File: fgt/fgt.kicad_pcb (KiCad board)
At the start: 2 copper layers, 78 x 78 mm, 60 parts, among them J1 Conn_01x02, J2 USB_B_Mini, J3 BL_Conn, J4 Conn_01x06, Q1 BC817, SW1 Reset, SW2 SW-, SW3 SW_M/BOOT, SW4 SW+, U1 ESP32-C3-WROOM-02, U2 ERC12864, U3 BMP280, U4 HT75xx-1-SOT89

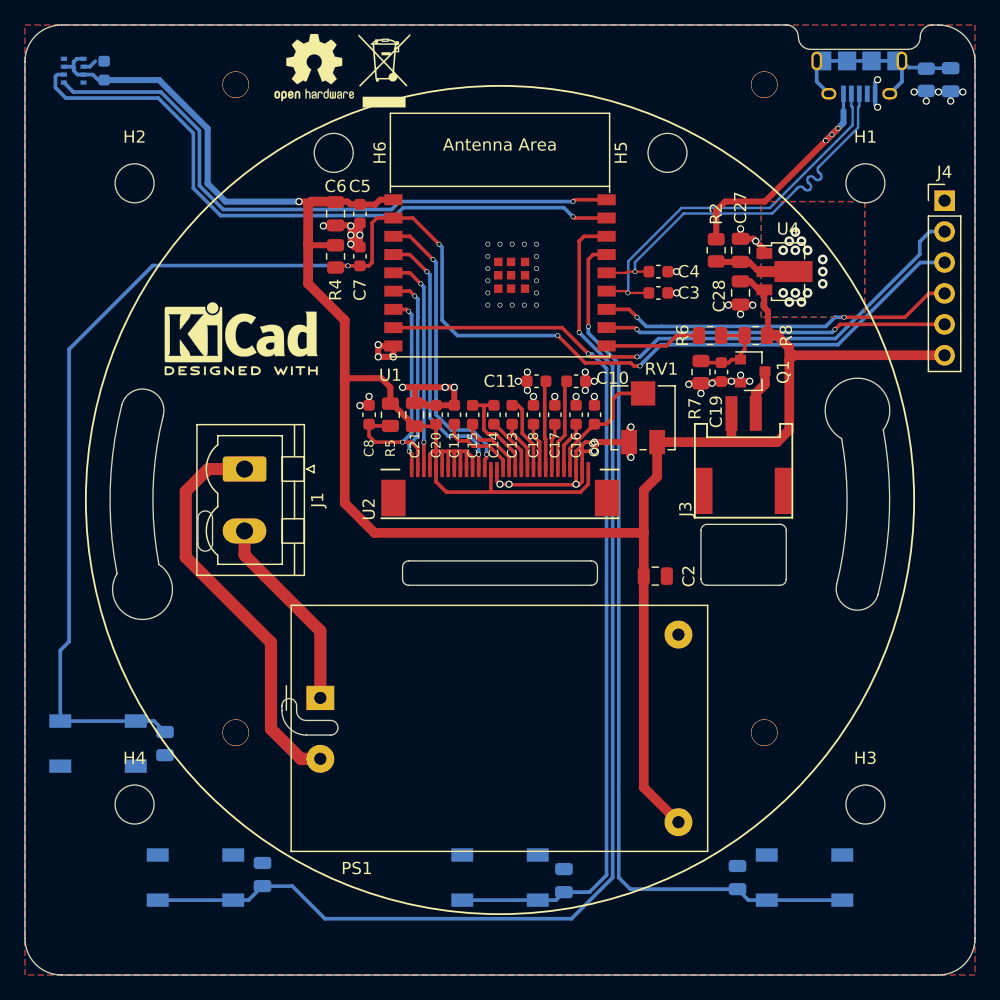
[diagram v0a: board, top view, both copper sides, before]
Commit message: retouch board layout v1.1.0
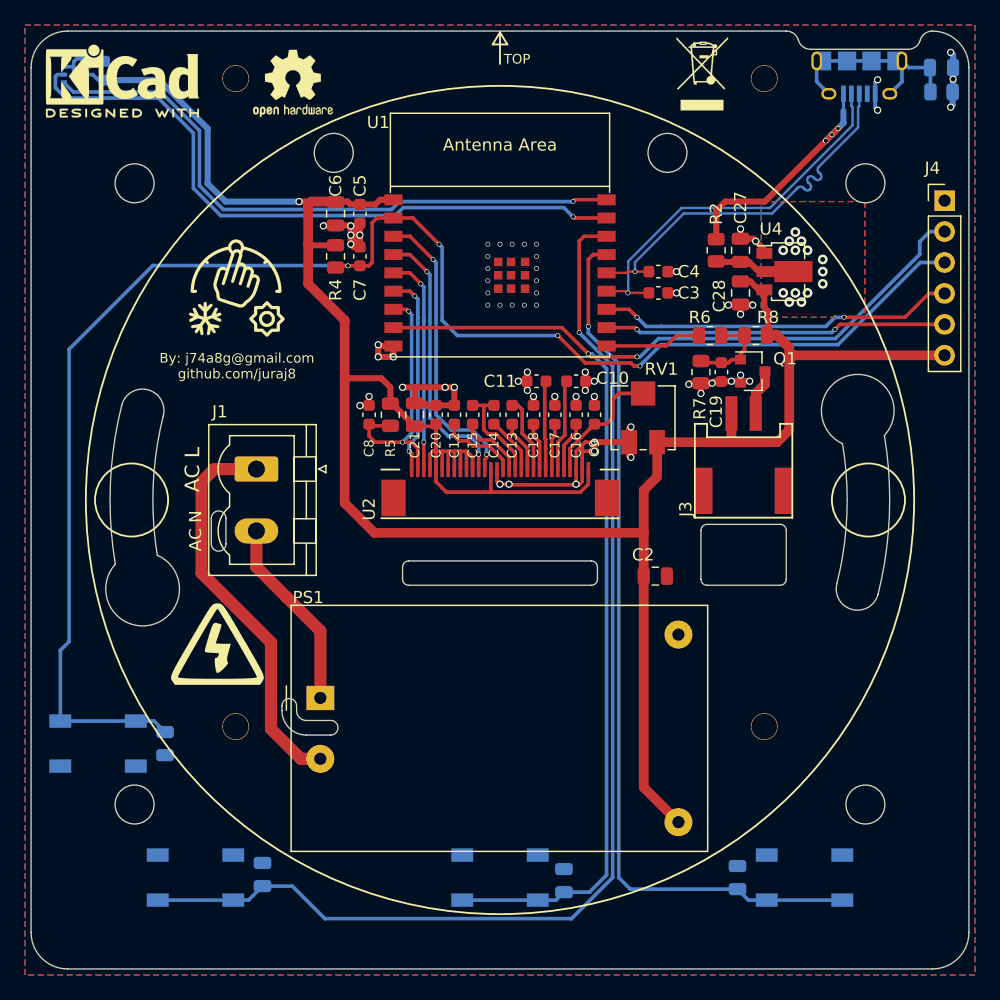
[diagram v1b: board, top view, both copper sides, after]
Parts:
- added G***: LOGO, LOGO, F.Cu at (98.4, 92.6)
- added G***: LOGO, LOGO, F.Cu at (96.8, 121.8)
- added G***: LOGO, LOGO, B.Cu at (112.6, 130.4)
- added G***: LOGO, LOGO, B.Cu at (153.6, 143.2)
- moved REF** 26.1 mm to (136.6, 75.0)
- moved REF** 23.3 mm to (89.0, 75.6)
- moved REF** 2.18 mm to (103.0, 75.8)
- moved R1 1.60 mm to (156.2, 76.5), turned to 0 degrees
- moved C1 1.25 mm to (156.2, 74.5), turned to 0 degrees
- moved J1 0.97 mm to (100.0, 107.5)
- moved Display 0.50 mm to (120.0, 102.0)
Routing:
- net GND: track 80.5 -> 79.6 mm, vias 68 -> 66
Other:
- board size 78 x 78 mm -> 77 x 77 mm
- board text added: "AC L"
- board text added: "AC N"
- board text added: "BOOT ENABLE TXD RXD 3V3"
- board text added: "By: j74a8g@gmail.com github.com/juraj8"
- board text added: "FGT"
- board text added: "Jan 2021. Rev 1.1.0"
- board text added: "TOP"
